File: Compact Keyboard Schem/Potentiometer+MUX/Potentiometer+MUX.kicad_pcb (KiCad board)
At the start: 2 copper layers, 66 x 157 mm, 16 parts, among them J1 Conn_01x04, J2 Conn_01x02, J3 Conn_01x08, J4 Conn_01x16

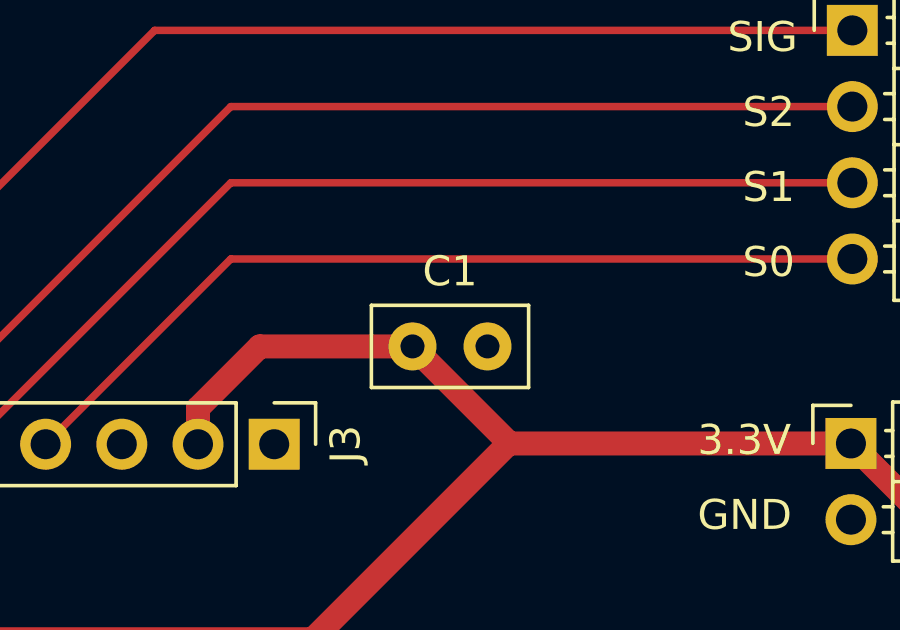
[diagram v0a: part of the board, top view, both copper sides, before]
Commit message: Pushing Update
Latest version after PCB printing
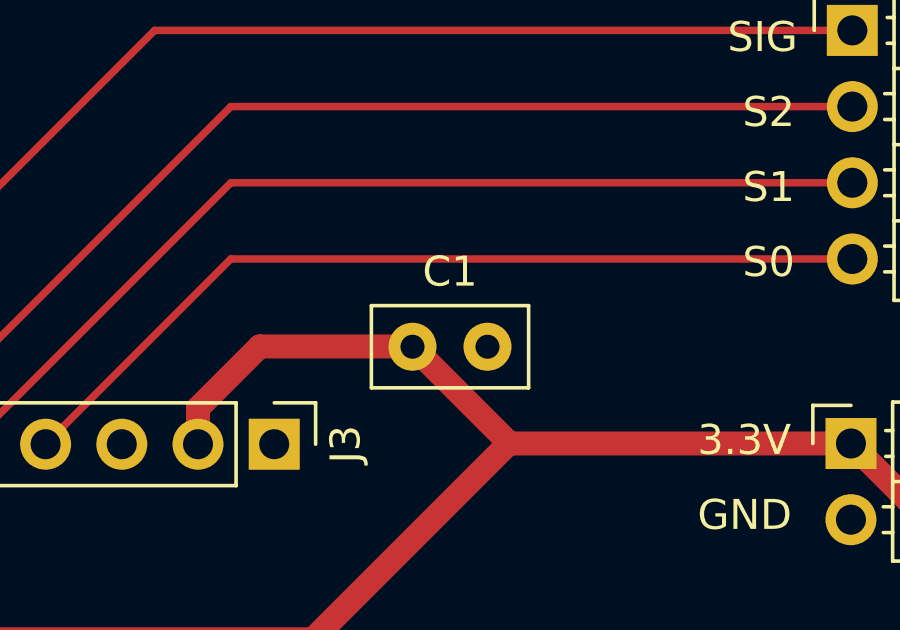
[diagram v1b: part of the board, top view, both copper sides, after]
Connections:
- J3 pad 7: unconnected-(J3-Pin_7-Pad7) -> GND
